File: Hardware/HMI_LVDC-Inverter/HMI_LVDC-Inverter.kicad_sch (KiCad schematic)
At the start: 1 part, among them J10 Conn_01x06_Pin

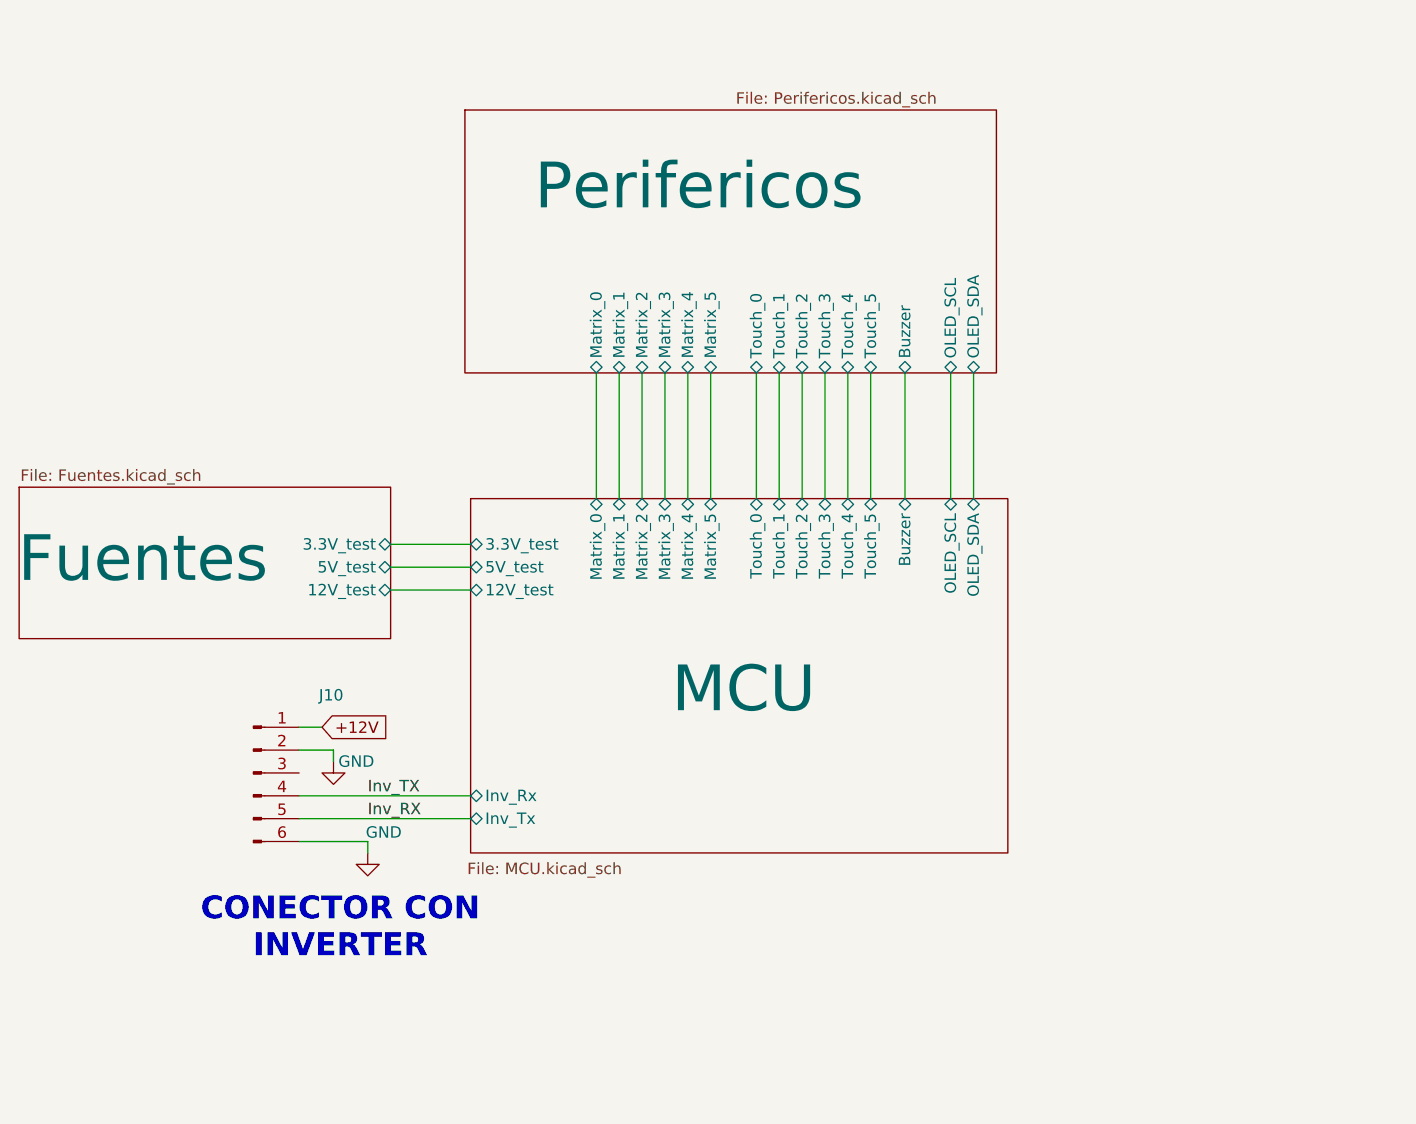
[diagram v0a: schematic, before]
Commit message: Terminado el esquemático del HMI
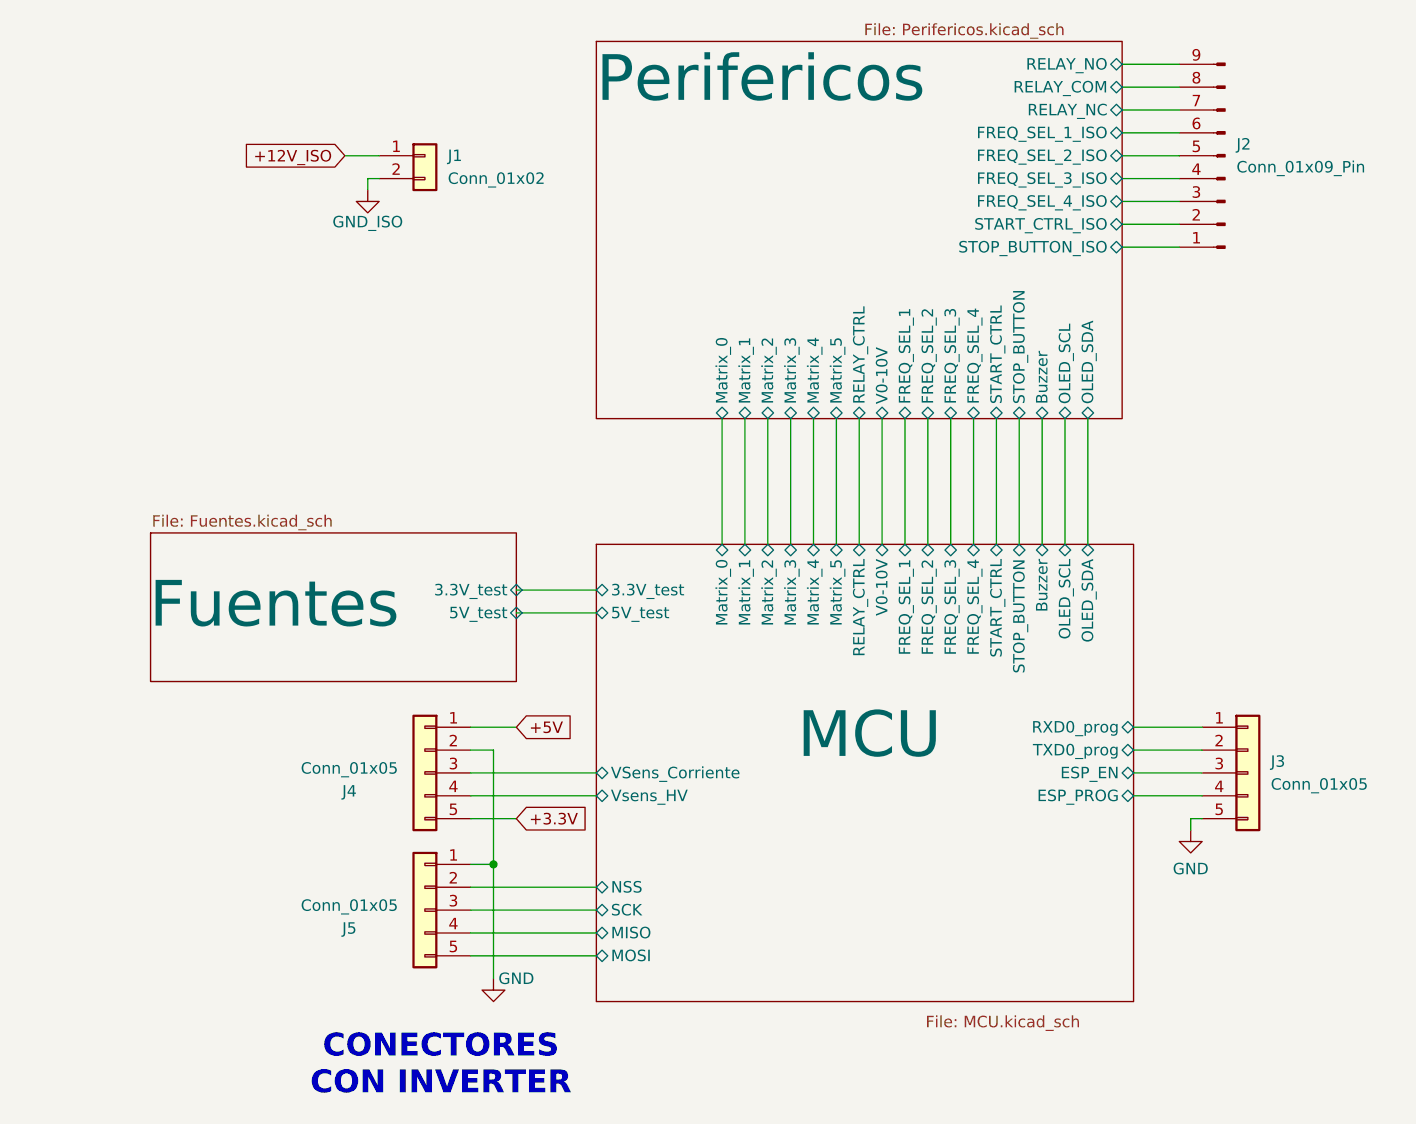
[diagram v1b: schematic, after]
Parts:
- removed J10: Conn_01x06_Pin, symbol Connector:Conn_01x06_Pin
- added J1: Conn_01x02, Connector_Hirose:Hirose_DF13-02P-1.25DS_1x02_P1.25mm_Horizontal, symbol Connector_Generic:Conn_01x02
- added J2: Conn_01x09_Pin, Connector_Phoenix_SPT:PhoenixContact_SPT_2.5_9-V-5.0-EX_1x09_P5.0mm_Vertical, symbol Connector:Conn_01x09_Pin
- added J3, J4, J5: Conn_01x05, Connector_PinHeader_1.00mm:PinHeader_1x05_P1.00mm_Vertical, symbol Connector_Generic:Conn_01x05
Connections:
- net GND: now also J3.5 (Pin_5), J4.2 (Pin_2), J5.1 (Pin_1)
- new net +12V_ISO: J1.1 (Pin_1)
- new net +3.3V: J4.5 (Pin_5)
- new net +5V: J4.1 (Pin_1)
- new net GND_ISO: J1.2 (Pin_2)
- new net MCU/ESP_EN: J3.3 (Pin_3)
- new net MCU/ESP_PROG: J3.4 (Pin_4)
- new net MCU/MISO: J5.4 (Pin_4)
- new net MCU/MOSI: J5.5 (Pin_5)
- new net MCU/NSS: J5.2 (Pin_2)
- new net MCU/RXD0_prog: J3.1 (Pin_1)
- new net MCU/SCK: J5.3 (Pin_3)
- new net MCU/TXD0_prog: J3.2 (Pin_2)
- new net MCU/VSens_Corriente: J4.3 (Pin_3)
- new net MCU/Vsens_HV: J4.4 (Pin_4)
- new net Perifericos/FREQ_SEL_1_ISO: J2.6 (Pin_6)
- new net Perifericos/FREQ_SEL_2_ISO: J2.5 (Pin_5)
- new net Perifericos/FREQ_SEL_3_ISO: J2.4 (Pin_4)
- new net Perifericos/FREQ_SEL_4_ISO: J2.3 (Pin_3)
- new net Perifericos/RELAY_COM: J2.8 (Pin_8)
- new net Perifericos/RELAY_NC: J2.7 (Pin_7)
- new net Perifericos/RELAY_NO: J2.9 (Pin_9)
- new net Perifericos/START_CTRL_ISO: J2.2 (Pin_2)
- new net Perifericos/STOP_BUTTON_ISO: J2.1 (Pin_1)
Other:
- sheet Fuentes ports: added none; removed 12V_test
- sheet MCU ports: added ESP_EN, ESP_PROG, FREQ_SEL_1, FREQ_SEL_2, FREQ_SEL_3, FREQ_SEL_4, MISO, MOSI, NSS, RELAY_CTRL, RXD0_prog, SCK, START_CTRL, STOP_BUTTON, TXD0_prog, V0-10V, VSens_Corriente, Vsens_HV; removed 12V_test, Inv_Rx, Inv_Tx, Touch_0, Touch_1, Touch_2, Touch_3, Touch_4, Touch_5
- sheet Perifericos ports: added FREQ_SEL_1, FREQ_SEL_1_ISO, FREQ_SEL_2, FREQ_SEL_2_ISO, FREQ_SEL_3, FREQ_SEL_3_ISO, FREQ_SEL_4, FREQ_SEL_4_ISO, RELAY_COM, RELAY_CTRL, RELAY_NC, RELAY_NO, START_CTRL, START_CTRL_ISO, STOP_BUTTON, STOP_BUTTON_ISO, V0-10V; removed Touch_0, Touch_1, Touch_2, Touch_3, Touch_4, Touch_5
- note added: "CONECTORES CON INVERTER"
- note removed: "CONECTOR CON INVERTER"
